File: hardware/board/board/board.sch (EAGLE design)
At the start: 2 parts, among them M1 WIRELESS-NRF24L01

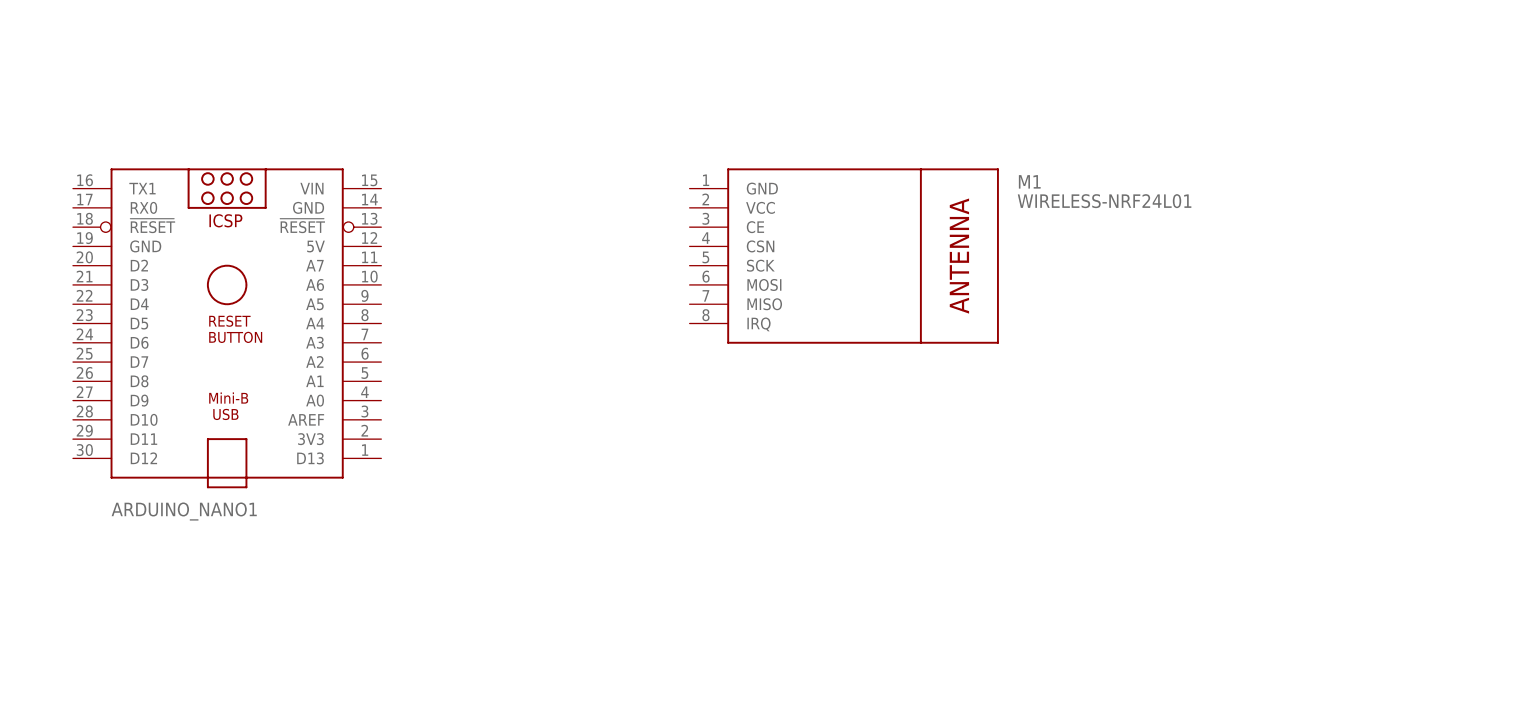
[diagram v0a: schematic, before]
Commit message: added schematic and board files
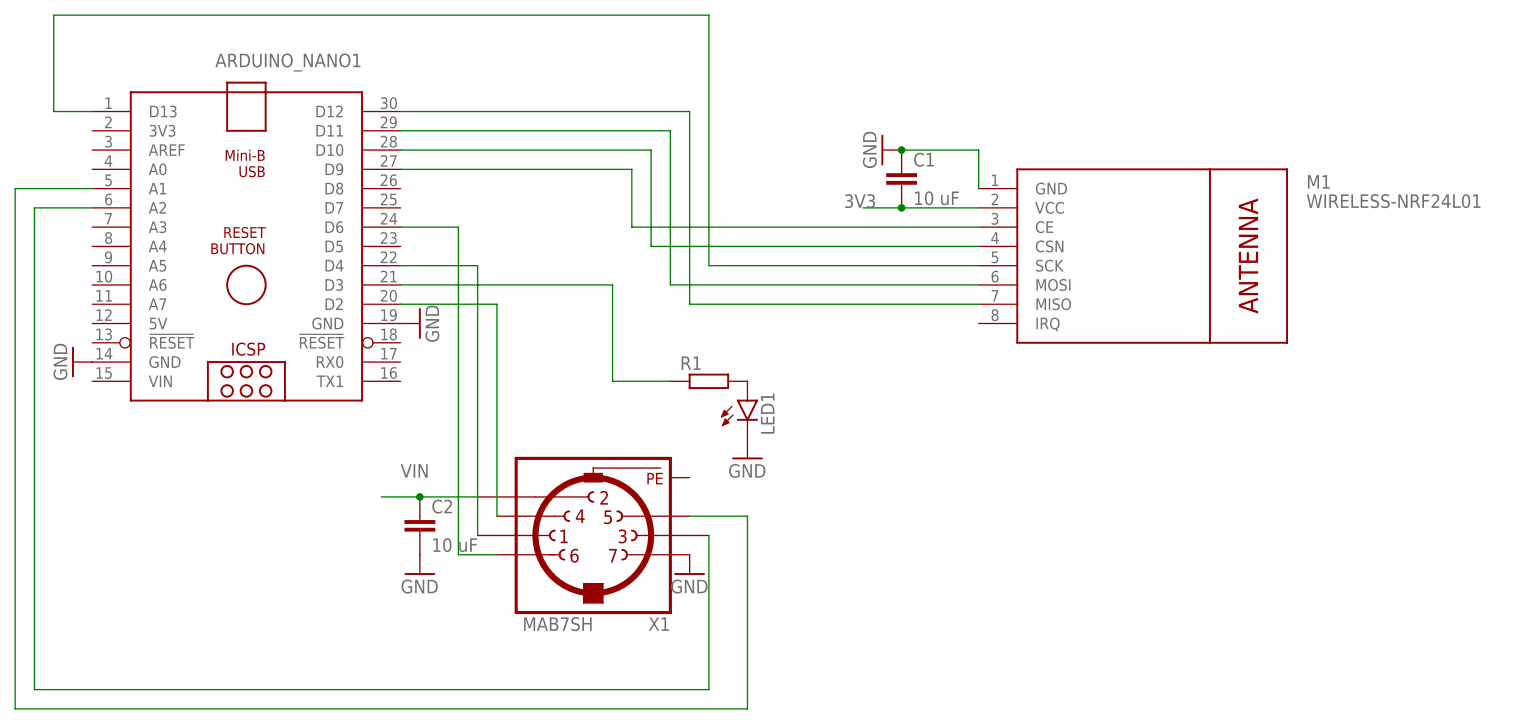
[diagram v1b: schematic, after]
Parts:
- added C1, C2: 10 uF, rcl:C-EUC0805
- added LED1: (no value), led:LED5MM
- added R1: (no value), rcl:R-EU_R0805
- added X1: MAB7SH, con-hirschmann:MAB7SH
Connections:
- new net 3V3: C1.2, M1.VCC
- new net GND: ARDUINO_NANO1.GND@1, ARDUINO_NANO1.GND@2, C1.1, C2.2, LED1.C, M1.GND, X1.7
- new net N$1: ARDUINO_NANO1.D13, M1.SCK
- new net N$10: ARDUINO_NANO1.D4, X1.1
- new net N$11: ARDUINO_NANO1.A1, X1.5
- new net N$12: ARDUINO_NANO1.D2, X1.4
- new net N$2: ARDUINO_NANO1.D12, M1.MISO
- new net N$3: ARDUINO_NANO1.D11, M1.MOSI
- new net N$4: ARDUINO_NANO1.D10, M1.CSN
- new net N$5: ARDUINO_NANO1.D9, M1.CE
- new net N$6: LED1.A, R1.2
- new net N$7: ARDUINO_NANO1.D3, R1.1
- new net N$8: ARDUINO_NANO1.D6, X1.6
- new net N$9: ARDUINO_NANO1.A2, X1.3
- new net VIN: C2.1, X1.2
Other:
- moved on the sheet: ARDUINO_NANO1, M1
